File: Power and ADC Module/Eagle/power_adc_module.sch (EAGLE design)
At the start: 11 parts

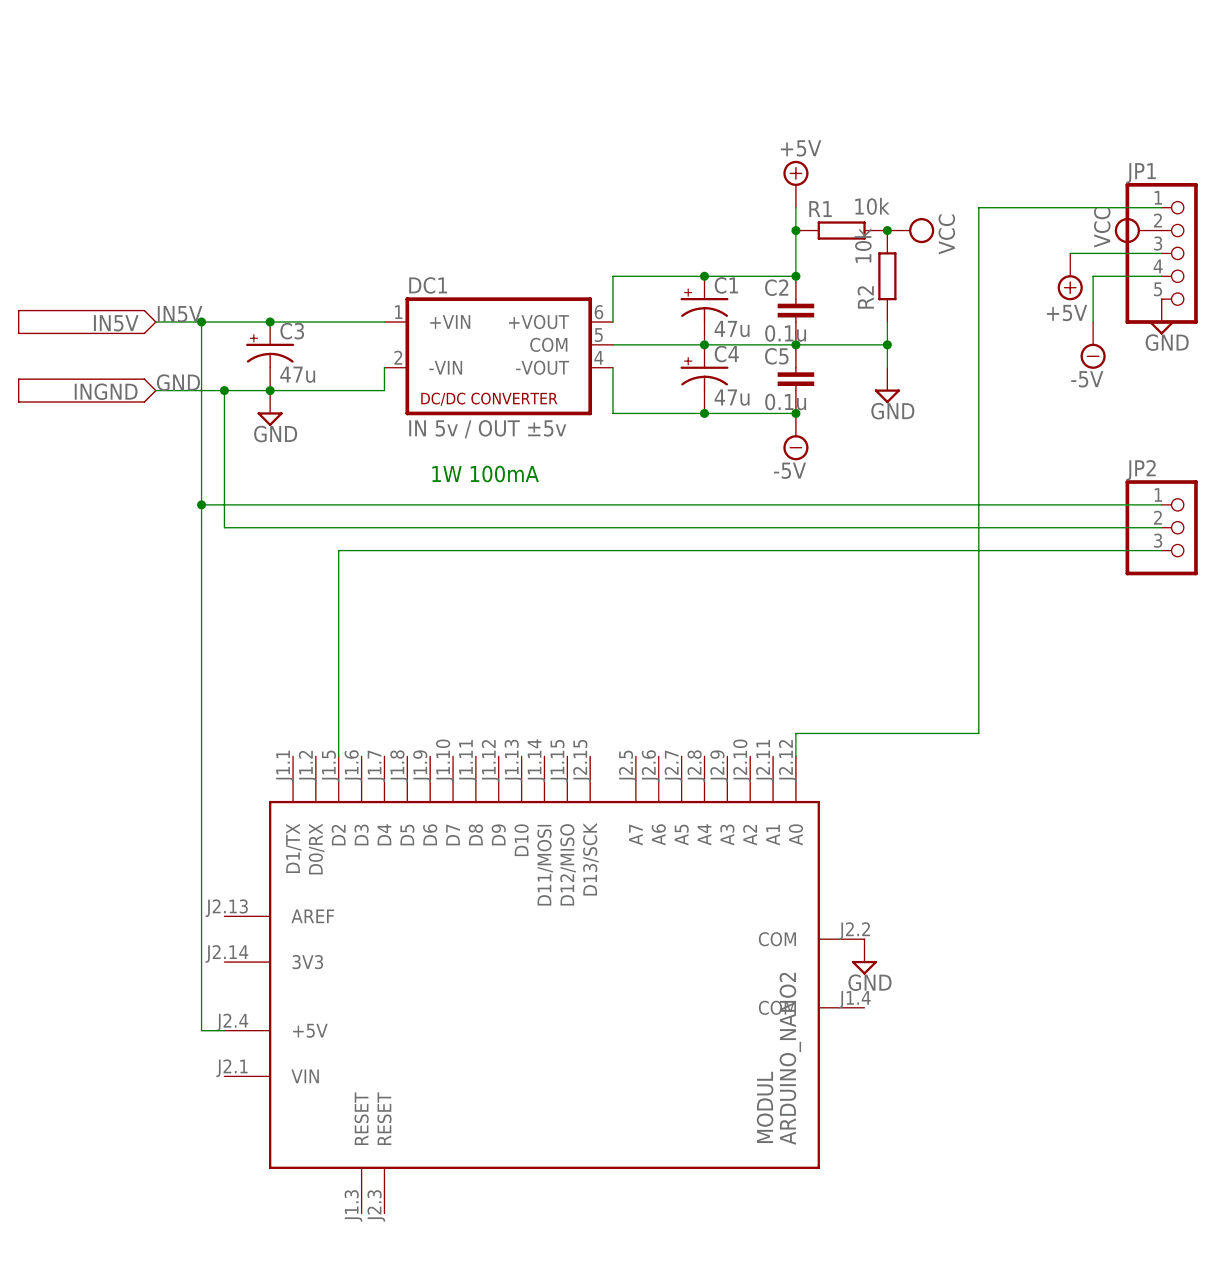
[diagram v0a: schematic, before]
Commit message: Update: v1.1.0
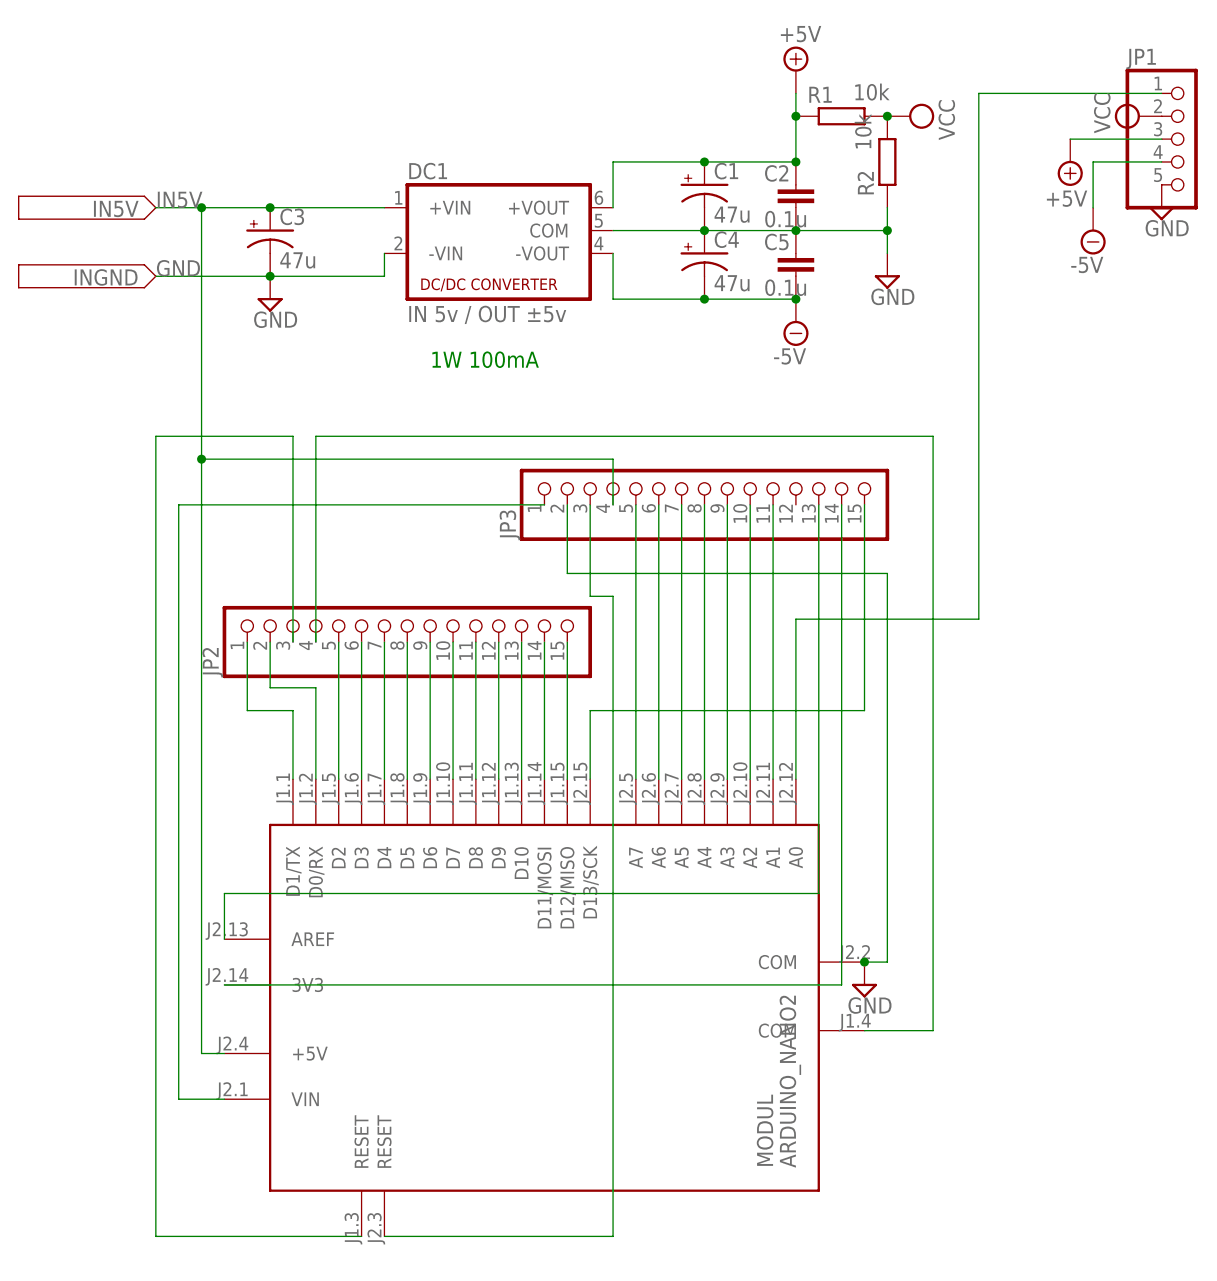
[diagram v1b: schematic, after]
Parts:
- added JP3: (no value), pinhead:PINHD-1X15
- JP2: device pinhead:PINHD-1X3 -> pinhead:PINHD-1X15
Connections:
- new net N$10: JP2.9, MODUL.D6
- new net N$11: JP2.10, MODUL.D7
- new net N$12: JP2.11, MODUL.D8
- new net N$13: JP2.12, MODUL.D9
- new net N$14: JP2.13, MODUL.D10
- new net N$15: JP2.14, MODUL.D11/MOSI
- new net N$16: JP2.15, MODUL.D12/MISO
- new net N$17: JP3.1, MODUL.VIN
- new net N$18: JP3.3, MODUL.RESET@2
- new net N$19: JP3.5, MODUL.A7
- new net N$2: JP2.2, MODUL.D0/RX
- new net N$20: JP3.6, MODUL.A6
- new net N$21: JP3.7, MODUL.A5
- new net N$22: JP3.8, MODUL.A4
- new net N$23: JP3.9, MODUL.A3
- new net N$24: JP3.10, MODUL.A2
- new net N$25: JP3.11, MODUL.A1
- new net N$26: JP3.15, MODUL.D13/SCK
- new net N$27: JP3.13, MODUL.AREF
- new net N$28: JP3.14, MODUL.3V3
- new net N$4: JP2.3, MODUL.RESET
- new net N$5: JP2.4, MODUL.COM
- new net N$6: JP2.5, MODUL.D2
- new net N$7: JP2.6, MODUL.D3
- new net N$8: JP2.7, MODUL.D4
- new net N$9: JP2.8, MODUL.D5
- net GND: now also JP3.2; no longer JP2.2
- net IN5V: now also JP3.4; no longer JP2.1
- net N$3: now also JP2.1, MODUL.D1/TX; no longer JP2.3, MODUL.D2
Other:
- moved on the sheet: C1, C2, C3, C4, C5, DC1, JP1, MODUL, R1, R2
